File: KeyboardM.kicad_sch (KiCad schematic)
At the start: 21 parts, among them J1 AVR-ISP-6, U1 ATmega32U4-A, U2 PRTR5V0U2X, Y1 Crystal_GND24_Small

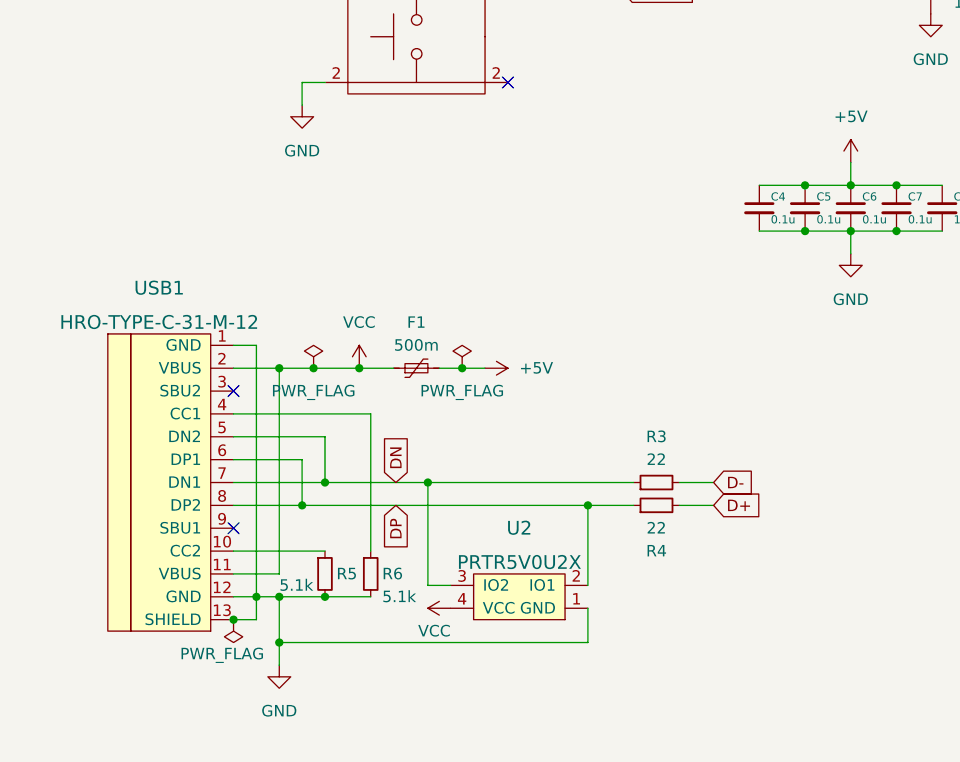
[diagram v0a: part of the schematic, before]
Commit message: v1.0.0
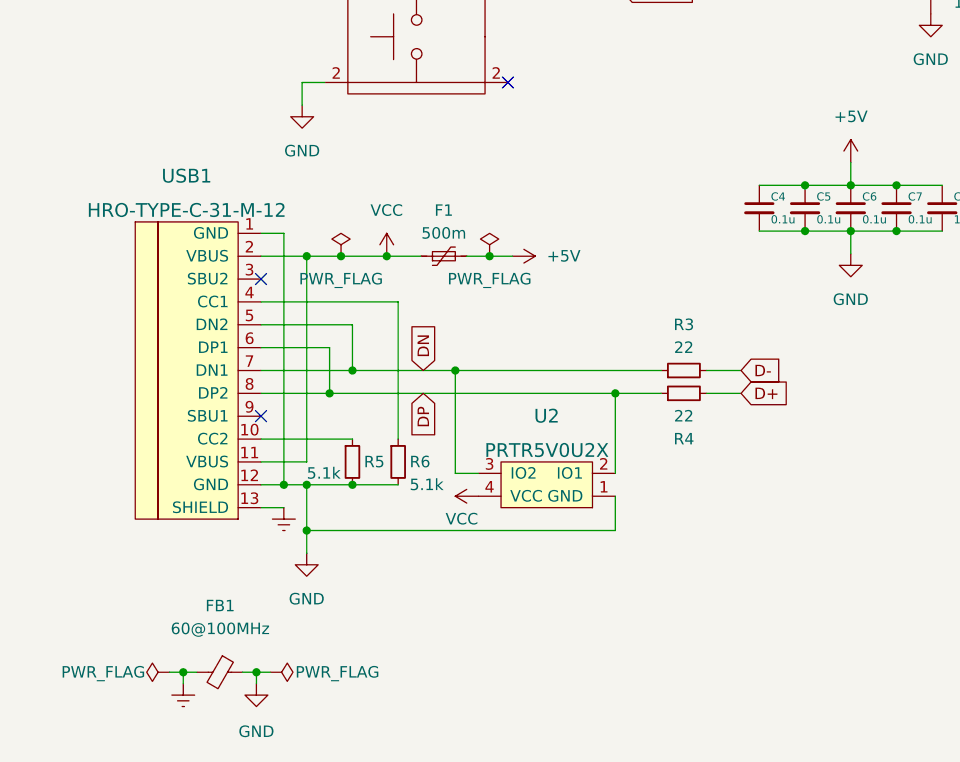
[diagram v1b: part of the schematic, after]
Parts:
- added FB1: 60@100MHz, Inductor_SMD:L_0805_2012Metric_Pad1.15x1.40mm_HandSolder, symbol Device:FerriteBead_Small
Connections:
- net GND: now also FB1.1; no longer USB1.13 (SHIELD)
- new net Earth: FB1.2, USB1.13 (SHIELD)
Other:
- moved on the sheet: F1, R3, R4, R5, R6, U2, USB1
